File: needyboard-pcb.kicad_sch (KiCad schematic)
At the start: 9 parts, among them U1 ProMicro

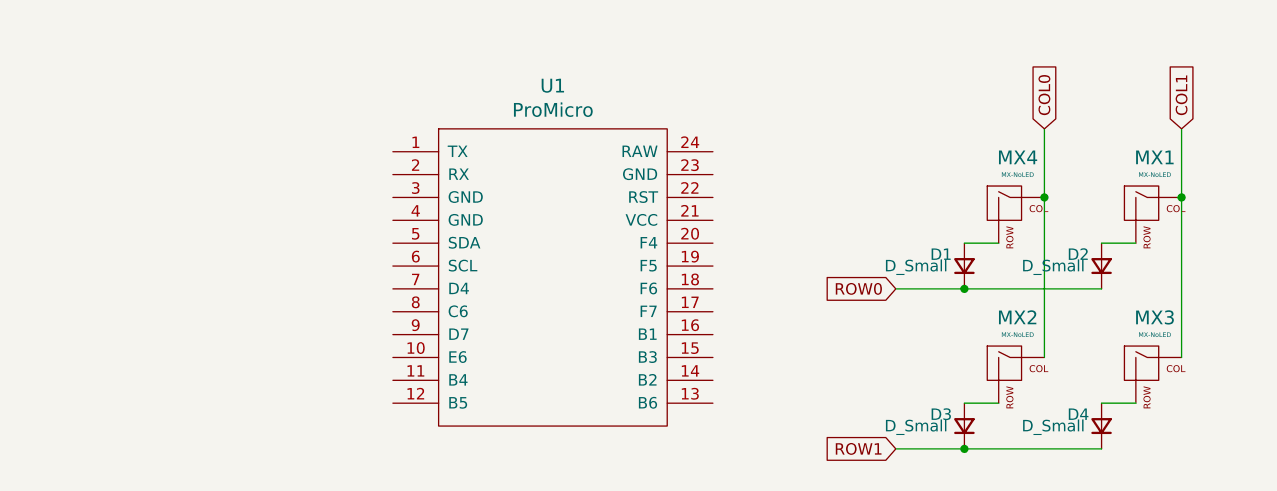
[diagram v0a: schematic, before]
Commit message: complete
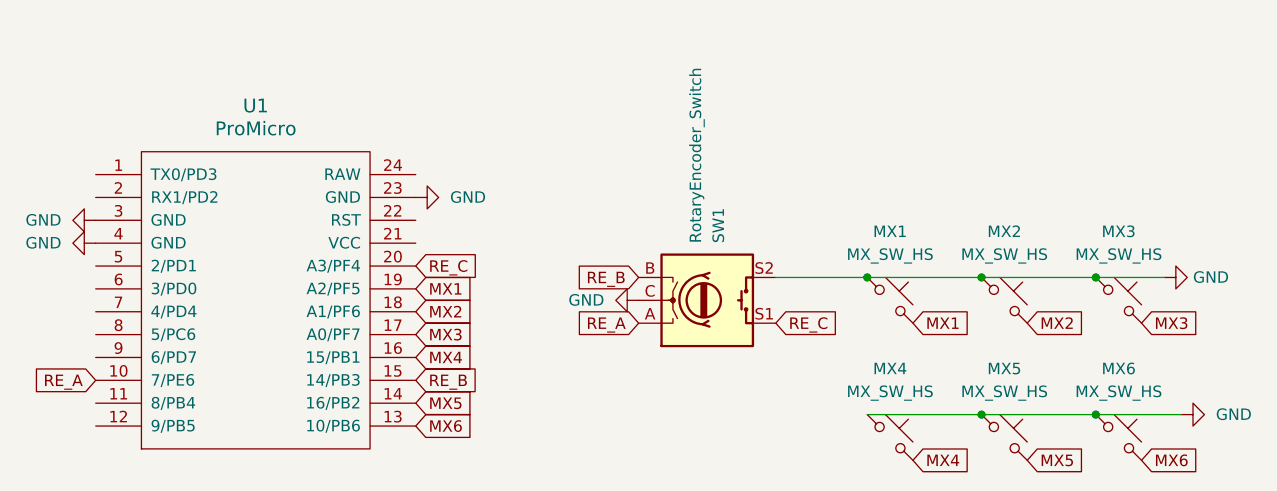
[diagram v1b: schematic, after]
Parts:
- removed D1, D2, D3, D4: D_Small, Diode_SMD:D_SOD-123, symbol Device:D_Small
- removed MX1, MX2, MX3, MX4: MX-NoLED, Button_Switch_Keyboard:SW_Cherry_MX_1.00u_PCB, symbol MX_Alps_Hybrid:MX-NoLED
- removed U1: ProMicro, promicro:ProMicro, symbol promicro:ProMicro
- added MX1, MX2, MX3, MX4, MX5, MX6: MX_SW_HS, PCM_marbastlib-mx:SW_MX_HS_1u, symbol PCM_marbastlib-mx:MX_SW_HS
- added SW1: RotaryEncoder_Switch, Keebio-Parts.pretty-master:RotaryEncoder_EC11, symbol Device:RotaryEncoder_Switch
- added U1: ProMicro, Keebio-Parts.pretty-master:ArduinoProMicro, symbol keebio:ProMicro
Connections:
- new net GND: MX1.1, MX2.1, MX3.1, MX4.1, MX5.1, MX6.1, SW1.C, SW1.S2, U1.23 (GND), U1.3 (GND), U1.4 (GND)
- new net MX1: MX1.2, U1.19 (A2/PF5)
- new net MX2: MX2.2, U1.18 (A1/PF6)
- new net MX3: MX3.2, U1.17 (A0/PF7)
- new net MX4: MX4.2, U1.16 (15/PB1)
- new net MX5: MX5.2, U1.14 (16/PB2)
- new net MX6: MX6.2, U1.13 (10/PB6)
- new net RE_A: SW1.A, U1.10 (7/PE6)
- new net RE_B: SW1.B, U1.15 (14/PB3)
- new net RE_C: SW1.S1, U1.20 (A3/PF4)
